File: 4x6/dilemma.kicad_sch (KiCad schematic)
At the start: 330 parts, among them J1 USB_C_Receptacle_USB2.0, J102 NA_serial, J105 NA_Conn_01x04_Female, J113 Cirque, J3 NA_GC9A01, J4 Conn_01x05, J5 NA_Conn_01x02, J5001 USB_C_Receptacle_USB2.0, J5002 NA_Conn_01x02, J5003 NA_serial, J5004 NA_GC9A01, J5005 NA_Conn_01x04_Female, J5007 Cirque, J5008 Conn_01x05, J5009 Conn_01x05, J5010 Conn_01x05, SW1 SW_Push, SW101 NA_SW_Push, SW102 NA_SW_Push, SW103 NA_SW_Push, SW104 NA_SW_Push, SW105 NA_SW_Push, SW106 NA_SW_Push, SW107 NA_SW_Push, SW108 NA_SW_Push, SW109 NA_SW_Push, SW112 NA_SW_Push, SW113 NA_SW_Push, SW114 NA_SW_Push, SW115 NA_SW_Push, SW116 NA_SW_Push, SW117 NA_SW_Push, SW118 NA_SW_Push, SW119 NA_SW_Push, SW3001 NA_SW_Push, SW3002 NA_RotaryEncoder_Switch, SW5001 SW_Push, SW5002 NA_SW_Push, SW5003 NA_SW_Push, SW5004 NA_SW_Push, SW5005 NA_SW_Push, SW5006 NA_SW_Push, SW5007 NA_SW_Push, SW5008 NA_SW_Push, SW5009 NA_SW_Push, SW5010 NA_SW_Push, SW5011 NA_SW_Push, SW5012 NA_SW_Push, SW5013 NA_SW_Push, SW5014 NA_SW_Push, SW5015 NA_SW_Push, SW5016 NA_SW_Push, SW5017 NA_SW_Push, SW5018 NA_SW_Push, SW5019 NA_SW_Push, SW5020 NA_RotaryEncoder_Switch, SW5021 SW_SPST, SW5022 SW_SPST, SW5023 NA_SW_Push, SW5024 NA_SW_Push, SW5025 NA_SW_Push, SW5026 NA_SW_Push, SW5027 NA_SW_Push, SW5028 NA_SW_Push, SW5029 NA_SW_Push, SW5030 NA_SW_Push, SW5031 NA_SW_Push, SW5032 NA_SW_Push, SW5033 NA_SW_Push, SW5034 NA_SW_Push, SW5035 NA_SW_Push, SW5036 NA_SW_Push, SW5037 NA_SW_Push, SW5038 NA_SW_Push, SW5039 NA_SW_Push, SW5040 NA_SW_Push, U1 RP2040, U2 W25Q128JVS, U3 XC6210B332MR-G, U4 USBLC6-2P6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

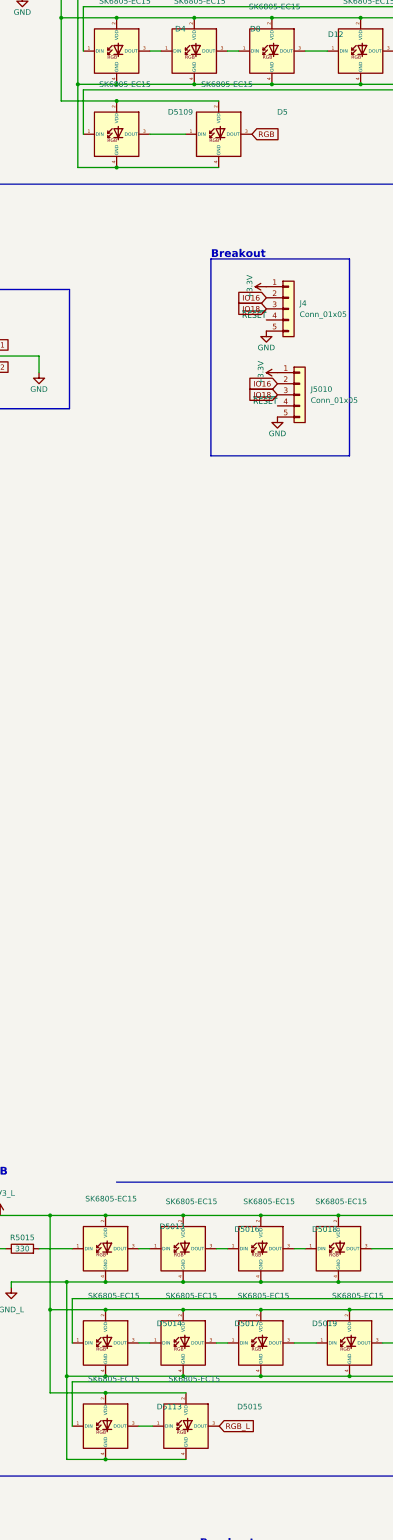
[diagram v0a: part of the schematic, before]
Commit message: routing
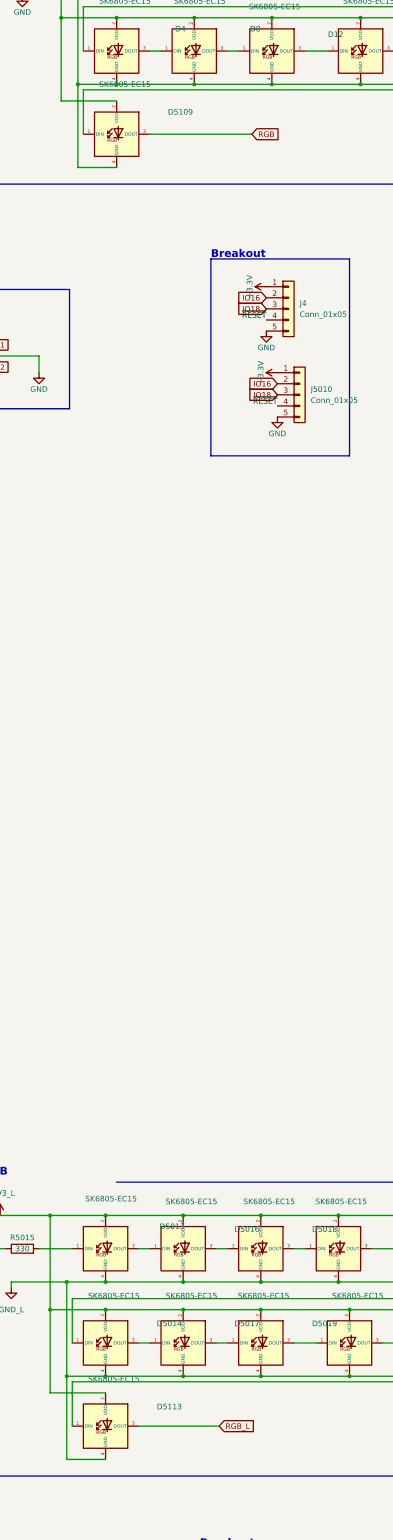
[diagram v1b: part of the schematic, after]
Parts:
- removed D5, D5015: SK6805-EC15, local-libraries:LED_SK6805-EC15_1.5x1.5mm_P0.6mm_handsolder, symbol sk6805-ec15:SK6805-EC15
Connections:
- net RGB: now also D5109.3 (DOUT)
- net RGB_L: now also D5113.3 (DOUT)
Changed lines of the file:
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@@
   (junction (at 241.3 414.655) (diameter 0) (color 0 0 0 0)
   )
-  (junction (at 402.59 67.31) (diameter 0) (color 0 0 0 0)
-  )
   (junction (at 148.59 185.42) (diameter 0) (color 0 0 0 0)
   )
@@
   (junction (at 402.59 48.26) (diameter 0) (color 0 0 0 0)
   )
-  (junction (at 402.59 82.55) (diameter 0) (color 0 0 0 0)
-  )
   (junction (at 130.81 185.42) (diameter 0) (color 0 0 0 0)
   )
@@
   (junction (at 438.15 48.26) (diameter 0) (color 0 0 0 0)
   )
-  (junction (at 400.05 378.46) (diameter 0) (color 0 0 0 0)
-  )
   (junction (at 455.93 41.91) (diameter 0) (color 0 0 0 0)
   )
@@
   (junction (at 120.65 524.51) (diameter 0) (color 0 0 0 0)
   )
-  (junction (at 400.05 363.22) (diameter 0) (color 0 0 0 0)
-  )
   (junction (at 402.59 26.67) (diameter 0) (color 0 0 0 0)
   )
@@
     (stroke (width 0) (type default))
   )
-  (wire (pts (xy 407.67 370.84) (xy 410.845 370.84))
+  (wire (pts (xy 407.67 370.84) (xy 426.085 370.84))
     (stroke (width 0) (type default))
   )
@@
     (stroke (width 0) (type default))
   )
-  (wire (pts (xy 402.59 67.31) (xy 425.958 67.31))
-    (stroke (width 0) (type default))
-  )
   (wire (pts (xy 116.84 518.16) (xy 116.84 528.32))
     (stroke (width 0) (type default))
@@
     (stroke (width 0) (type default))
   )
-  (wire (pts (xy 402.59 82.55) (xy 425.958 82.55))
-    (stroke (width 0) (type default))
-  )
   (wire (pts (xy 111.76 96.52) (xy 111.76 97.79))
     (stroke (width 0) (type default))
@@
     (stroke (width 0) (type default))
   )
-  (wire (pts (xy 400.05 378.46) (xy 418.465 378.46))
-    (stroke (width 0) (type default))
-  )
   (wire (pts (xy 721.995 128.905) (xy 732.155 128.905))
     (stroke (width 0) (type default))
@@
     (stroke (width 0) (type default))
   )
+  (wire (pts (xy 410.21 74.93) (xy 433.578 74.93))
+    (stroke (width 0) (type default))
+  )
   (wire (pts (xy 229.87 120.65) (xy 229.87 119.38))
     (stroke (width 0) (type default))
@@
     (stroke (width 0) (type default))
   )
-  (wire (pts (xy 410.21 74.93) (xy 418.338 74.93))
-    (stroke (width 0) (type default))
-  )
   (wire (pts (xy 127 220.98) (xy 127 218.44))
     (stroke (width 0) (type default))
@@
     (stroke (width 0) (type default))
   )
-  (wire (pts (xy 400.05 363.22) (xy 418.465 363.22))
-    (stroke (width 0) (type default))
-  )
   (polyline (pts (xy 346.075 462.28) (xy 372.745 462.28))
     (stroke (width 0) (type default))
@@
     )
   )
-  (symbol (lib_id "sk6805-ec15:SK6805-EC15") (at 425.958 74.93 0) (unit 1)
-    (in_bom yes) (on_board yes) (dnp no)
-    (property "Reference" "D5" (at 440.563 69.85 0)
-      (effects (font (size 1.27 1.27)))
-    )
-    (property "Value" "SK6805-EC15" (at 427.863 63.5 0)
-      (effects (font (size 1.27 1.27)))
-    )
-    (property "Footprint" "local-libraries:LED_SK6805-EC15_1.5x1.5mm_P0.6mm_handsolder" (at 427.228 82.55 0)
-      (effects (font (size 1.27 1.27)) (justify left top) hide)
-    )
-    (property "Datasheet" "https://datasheet.lcsc.com/lcsc/2108251530_OPSCO-Optoelectronics-SK6805-EC15_C2890035.pdf" (at 428.498 84.455 0)
-      (effects (font (size 1.27 1.27)) (justify left top) hide)
-    )
-    (property "MFN" "Dongguan Opsco Optoelectronics" (at 425.958 59.055 0)
-      (effects (font (size 1.27 1.27)) hide)
-    )
-    (property "MPN" "SK6805-EC15" (at 425.958 61.8301 0)
-      (effects (font (size 1.27 1.27)) hide)
-    )
-    (property "PKG" "SK6805-EC15" (at 425.958 64.6052 0)
-      (effects (font (size 1.27 1.27)) hide)
-    )
-    (property "LCSC" "C2890035" (at 425.958 74.93 0)
-      (effects (font (size 1.27 1.27)) hide)
-    )
-    (pin "1")
-    (pin "2")
-    (pin "3")
-    (pin "4")
-    (instances
-      (project "dilemma"
-        (path "/7353e96a-343a-4876-b497-b1d205a14d97"
-          (reference "D5") (unit 1)
-        )
-      )
-    )
-  )
   (symbol (lib_id "Device:D") (at 86.36 528.32 180) (unit 1)
     (in_bom yes) (on_board yes) (dnp no)
@@
         )
       )
-    )
-  )
-  (symbol (lib_id "sk6805-ec15:SK6805-EC15") (at 418.465 370.84 0) (unit 1)
-    (in_bom yes) (on_board yes) (dnp no)
-    (property "Reference" "D5015" (at 433.07 366.395 0)
-      (effects (font (size 1.27 1.27)))
-    )
-    (property "Value" "SK6805-EC15" (at 420.37 360.045 0)
-      (effects (font (size 1.27 1.27)))
-    )
-    (property "Footprint" "local-libraries:LED_SK6805-EC15_1.5x1.5mm_P0.6mm_handsolder" (at 419.735 378.46 0)
-      (effects (font (size 1.27 1.27)) (justify left top) hide)
-    )
-    (property "Datasheet" "https://datasheet.lcsc.com/lcsc/2108251530_OPSCO-Optoelectronics-SK6805-EC15_C2890035.pdf" (at 421.005 380.365 0)
-      (effects (font (size 1.27 1.27)) (justify left top) hide)
-    )
-    (property "MFN" "Dongguan Opsco Optoelectronics" (at 418.465 354.965 0)
-      (effects (font (size 1.27 1.27)) hide)
-    )
-    (property "MPN" "SK6805-EC15" (at 418.465 357.7401 0)
-      (effects (font (size 1.27 1.27)) hide)
-    )
-    (property "PKG" "SK6805-EC15" (at 418.465 360.5152 0)
-      (effects (font (size 1.27 1.27)) hide)
-    )
-    (property "LCSC" "C2890035" (at 418.465 370.84 0)
-      (effects (font (size 1.27 1.27)) hide)
-    )
-    (pin "1")
-    (pin "2")
-    (pin "3")
-    (pin "4")
-    (instances
-      (project "dilemma"
-        (path "/7353e96a-343a-4876-b497-b1d205a14d97"
-          (reference "D5015") (unit 1)
-        )
-      )

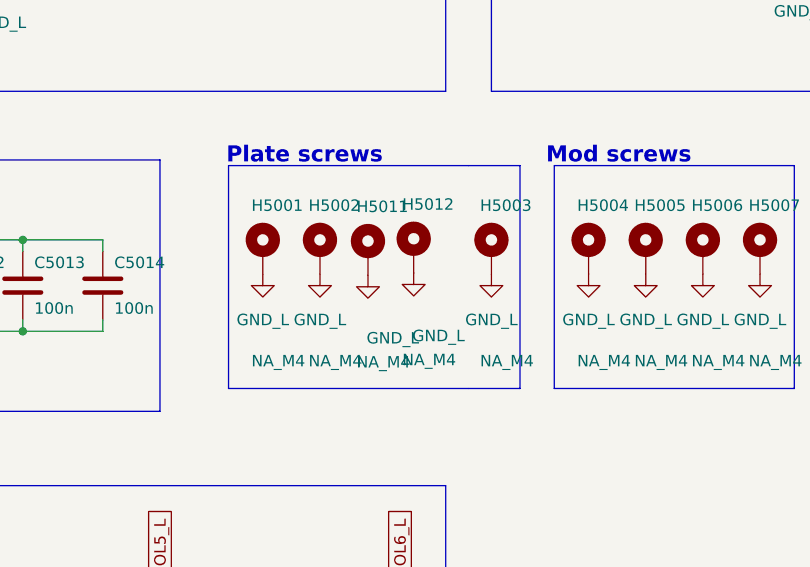
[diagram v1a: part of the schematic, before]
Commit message: routing
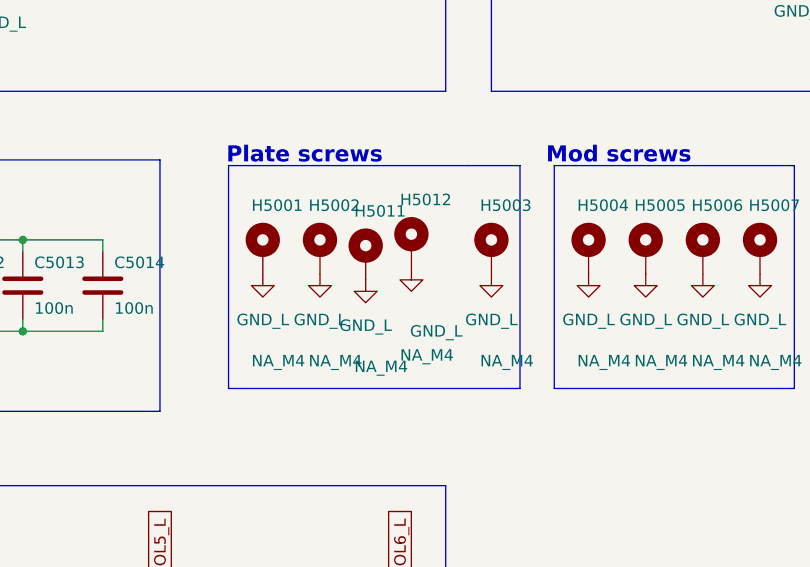
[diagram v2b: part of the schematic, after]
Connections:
- net GND: no longer H5011.1
- net GND_L: now also H5011.1
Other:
- moved on the sheet: H5011
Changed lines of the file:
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@@
     )
   )
+  (symbol (lib_id "Mechanical:MountingHole_Pad") (at 198.12 471.17 0) (unit 1)
+    (in_bom yes) (on_board yes) (dnp no)
+    (property "Reference" "H5012" (at 196.85 466.09 0)
+      (effects (font (size 1.27 1.27)) (justify left))
+    )
+    (property "Value" "NA_M4" (at 196.85 483.362 0)
+      (effects (font (size 1.27 1.27)) (justify left))
+    )
+    (property "Footprint" "local-libraries:MountingHole_3mm_Pad_Via" (at 198.12 471.17 0)
+      (effects (font (size 1.27 1.27)) hide)
+    )
+    (property "Datasheet" "~" (at 198.12 471.17 0)
+      (effects (font (size 1.27 1.27)) hide)
+    )
+    (pin "1")
+    (instances
+      (project "dilemma"
+        (path "/7353e96a-343a-4876-b497-b1d205a14d97"
+          (reference "H5012") (unit 1)
+        )
+      )
+    )
+  )
   (symbol (lib_id "Device:C") (at 157.48 180.34 0) (unit 1)
     (in_bom yes) (on_board yes) (dnp no)
@@
     )
   )
-  (symbol (lib_id "Mechanical:MountingHole_Pad") (at 198.374 471.678 0) (unit 1)
-    (in_bom yes) (on_board yes) (dnp no)
-    (property "Reference" "H5012" (at 197.104 466.598 0)
-      (effects (font (size 1.27 1.27)) (justify left))
-    )
-    (property "Value" "NA_M4" (at 197.104 483.87 0)
-      (effects (font (size 1.27 1.27)) (justify left))
-    )
-    (property "Footprint" "local-libraries:MountingHole_3mm_Pad_Via" (at 198.374 471.678 0)
-      (effects (font (size 1.27 1.27)) hide)
-    )
-    (property "Datasheet" "~" (at 198.374 471.678 0)
-      (effects (font (size 1.27 1.27)) hide)
-    )
-    (pin "1")
-    (instances
-      (project "dilemma"
-        (path "/7353e96a-343a-4876-b497-b1d205a14d97"
-          (reference "H5012") (unit 1)
-        )
-      )
-    )
-  )
   (symbol (lib_id "Device:D") (at 199.39 222.25 180) (unit 1)
     (in_bom yes) (on_board yes) (dnp no)
@@
     )
   )
+  (symbol (lib_id "power_L:GND_L") (at 193.04 474.98 0) (unit 1)
+    (in_bom yes) (on_board yes) (dnp no) (fields_autoplaced)
+    (property "Reference" "#PWR05172" (at 193.04 481.33 0)
+      (effects (font (size 1.27 1.27)) hide)
+    )
+    (property "Value" "GND_L" (at 193.04 480.06 0)
+      (effects (font (size 1.27 1.27)))
+    )
+    (property "Footprint" "" (at 193.04 474.98 0)
+      (effects (font (size 1.27 1.27)) hide)
+    )
+    (property "Datasheet" "" (at 193.04 474.98 0)
+      (effects (font (size 1.27 1.27)) hide)
+    )
+    (pin "1")
+    (instances
+      (project "dilemma"
+        (path "/7353e96a-343a-4876-b497-b1d205a14d97"
+          (reference "#PWR05172") (unit 1)
+        )
+      )
+    )
+  )
   (symbol (lib_id "Device:R") (at 330.835 29.21 180) (unit 1)
     (in_bom yes) (on_board yes) (dnp no)
@@
     )
   )
-  (symbol (lib_id "power:GND") (at 198.374 474.218 0) (unit 1)
+  (symbol (lib_id "power:GND") (at 198.12 473.71 0) (unit 1)
     (in_bom yes) (on_board yes) (dnp no)
-    (property "Reference" "#PWR05173" (at 198.374 480.568 0)
+    (property "Reference" "#PWR05173" (at 198.12 480.06 0)
       (effects (font (size 1.27 1.27)) hide)
     )
-    (property "Value" "GND_L" (at 198.218 481.2029 0)
+    (property "Value" "GND_L" (at 197.964 480.6949 0)
       (effects (font (size 1.27 1.27)) (justify left))
     )
-    (property "Footprint" "" (at 198.374 474.218 0)
+    (property "Footprint" "" (at 198.12 473.71 0)
       (effects (font (size 1.27 1.27)) hide)
     )
-    (property "Datasheet" "" (at 198.374 474.218 0)
+    (property "Datasheet" "" (at 198.12 473.71 0)
       (effects (font (size 1.27 1.27)) hide)
     )
@@
     )
   )
-  (symbol (lib_id "power:GND") (at 193.294 474.472 0) (unit 1)
-    (in_bom yes) (on_board yes) (dnp no)
-    (property "Reference" "#PWR05172" (at 193.294 480.822 0)
-      (effects (font (size 1.27 1.27)) hide)
-    )
-    (property "Value" "GND_L" (at 193.138 481.4569 0)
-      (effects (font (size 1.27 1.27)) (justify left))
-    )
-    (property "Footprint" "" (at 193.294 474.472 0)
-      (effects (font (size 1.27 1.27)) hide)
-    )
-    (property "Datasheet" "" (at 193.294 474.472 0)
-      (effects (font (size 1.27 1.27)) hide)
-    )
-    (pin "1")
-    (instances
-      (project "dilemma"
-        (path "/7353e96a-343a-4876-b497-b1d205a14d97"
-          (reference "#PWR05172") (unit 1)
-        )
-      )
-    )
-  )
   (symbol (lib_id "Switch:SW_Push") (at 52.07 220.98 0) (unit 1)
     (in_bom yes) (on_board yes) (dnp no)
@@
     )
   )
-  (symbol (lib_id "Mechanical:MountingHole_Pad") (at 193.294 471.932 0) (unit 1)
+  (symbol (lib_id "Mechanical:MountingHole_Pad") (at 193.04 472.44 0) (unit 1)
     (in_bom yes) (on_board yes) (dnp no)
-    (property "Reference" "H5011" (at 192.024 466.852 0)
+    (property "Reference" "H5011" (at 191.77 467.36 0)
       (effects (font (size 1.27 1.27)) (justify left))
     )
-    (property "Value" "NA_M4" (at 192.024 484.124 0)
+    (property "Value" "NA_M4" (at 191.77 484.632 0)
       (effects (font (size 1.27 1.27)) (justify left))
     )
-    (property "Footprint" "local-libraries:MountingHole_3mm_Pad_Via" (at 193.294 471.932 0)
+    (property "Footprint" "local-libraries:MountingHole_3mm_Pad_Via" (at 193.04 472.44 0)
       (effects (font (size 1.27 1.27)) hide)
     )
-    (property "Datasheet" "~" (at 193.294 471.932 0)
+    (property "Datasheet" "~" (at 193.04 472.44 0)
       (effects (font (size 1.27 1.27)) hide)
     )
